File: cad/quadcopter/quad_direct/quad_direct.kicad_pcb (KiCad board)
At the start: 2 copper layers, 22.9 x 36.8 mm, 15 parts, among them SW1 SW_Push, SW2 SW_Push, U1 4pin_header, U2 8pin_header, U3 8pin_header, U4 3pin_header

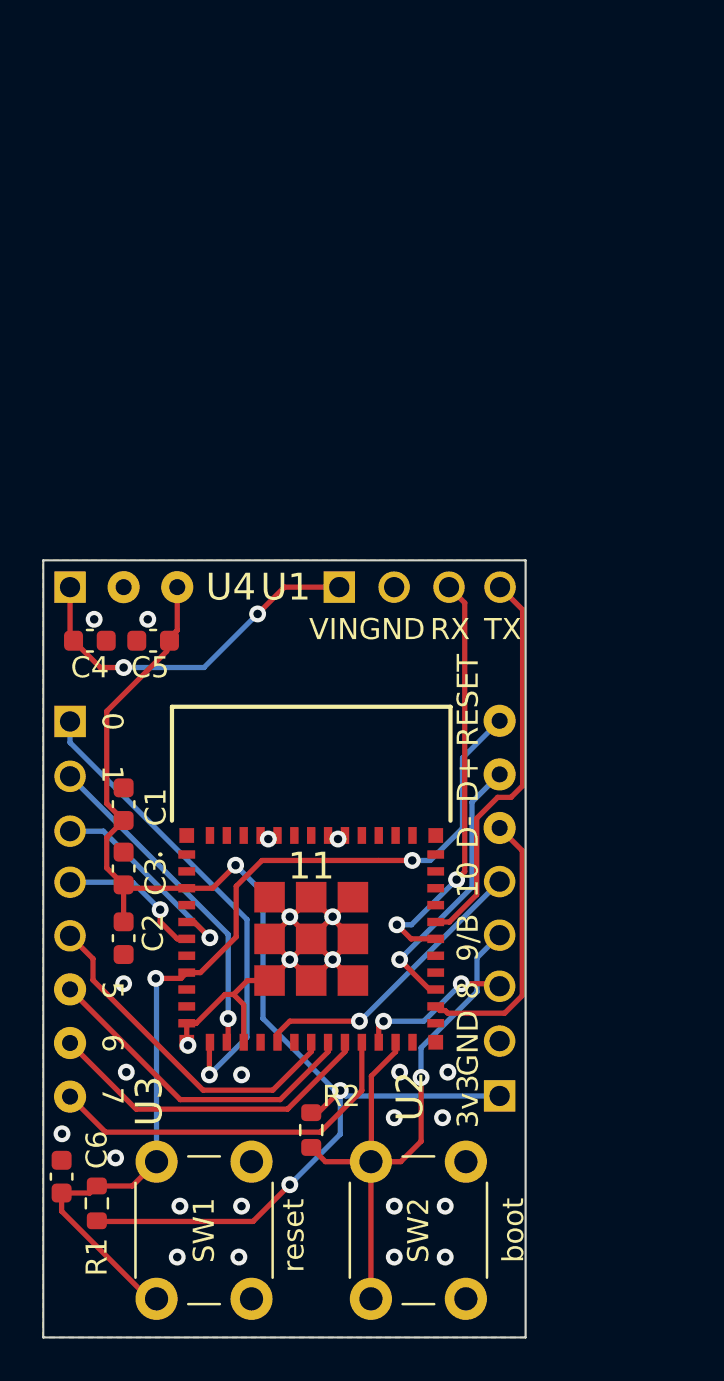
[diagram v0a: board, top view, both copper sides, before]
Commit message: Big progress saver
Signed-off-by: Andrew Wock <ajwock@gmail.com>
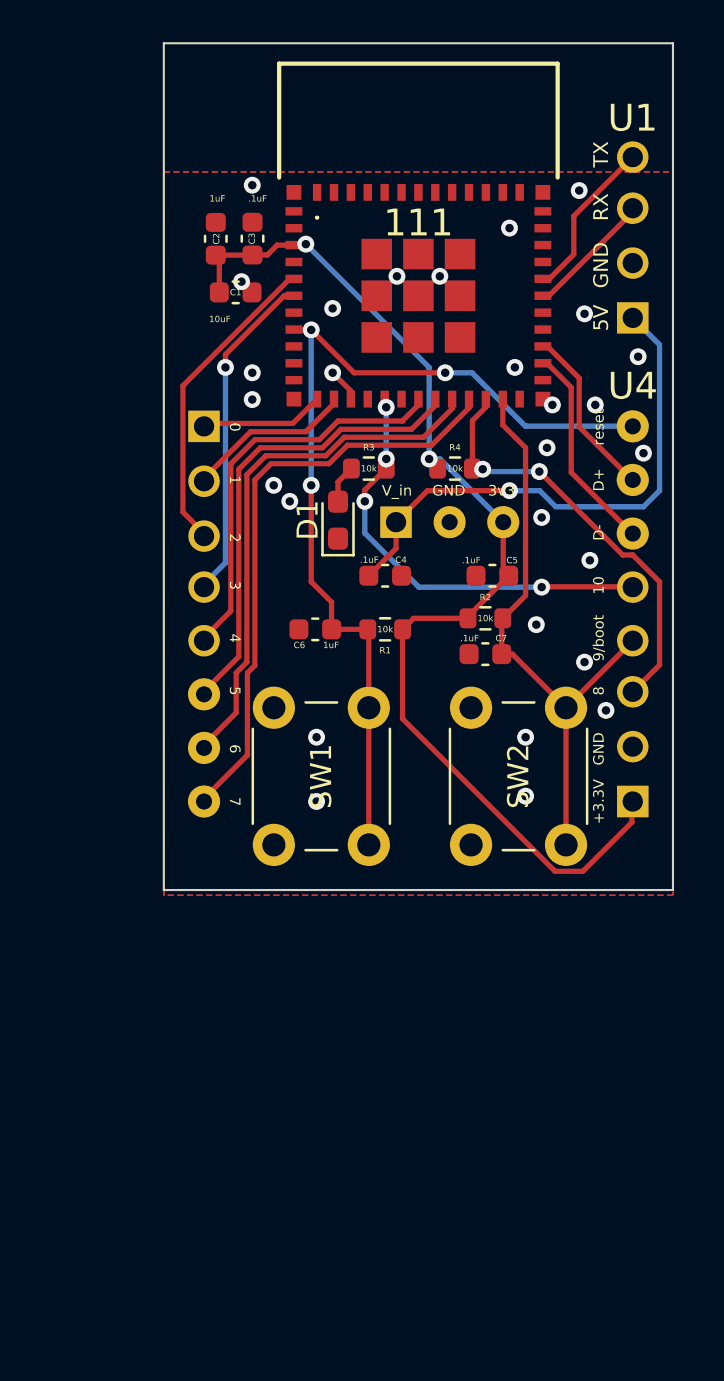
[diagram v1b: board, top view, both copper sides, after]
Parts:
- removed 11: ESP32-C3-MINI-1-H4X, Imported:ESP32C3MINI1H4X
- removed U3: 8pin_header, Imported:8-bb
- added 111: ESP32-C3-MINI-1-H4X, Imported:ESP32C3MINI1H4X, F.Cu at (165.1, 35.6)
- added C7: .1u, Capacitor_SMD:C_0603_1608Metric, F.Cu at (168.3, 55.2)
- added D1: LED, LED_SMD:LED_0603_1608Metric_Pad1.05x0.95mm_HandSolder, F.Cu at (161.3, 48.9)
- added R3: 10k, Resistor_SMD:R_0603_1608Metric, F.Cu at (162.8, 46.5)
- added R4: 10k, Resistor_SMD:R_0603_1608Metric, F.Cu at (166.8, 46.5)
- R1, R2: value R_US -> 10k
- U2: value 8pin_header -> esp32c3_boardout; footprint Imported:8-bb -> Imported:esp32c3_boardout
- moved C3 33.7 mm to (157.2, 35.6), turned to 90 degrees
- moved R1 30.4 mm to (163.5, 54.1), turned to 180 degrees
- moved C2 30.2 mm to (155.5, 35.6)
- moved SW1 29.8 mm to (162.8, 57.8), turned to -90 degrees
- moved SW2 29.5 mm to (172.1, 57.8), turned to -90 degrees
- moved C6 28.6 mm to (160.2, 54.1), turned to 180 degrees
- moved R2 25.6 mm to (168.3, 53.5), turned to 0 degrees
- moved C1 24.8 mm to (156.4, 38.1), turned to 0 degrees
- moved U2 20.9 mm to (152.4, 63.5), turned to 0 degrees
- moved U1 18.9 mm to (175.3, 39.3), turned to 90 degrees
- moved C5 16.4 mm to (168.6, 51.5)
- moved U4 15.8 mm to (164.0, 49.0)
- moved C4 14.3 mm to (163.5, 51.5)
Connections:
- U2 pad 1: +3V3 -> IO0
- U2 pad 2: GND -> IO1
- U2 pad 3: IO8 -> IO2
- U2 pad 4: IO9_BOOT -> IO3
- U2 pad 5: IO10 -> IO4
- U2 pad 6: IO18_USB_D- -> IO5
- U2 pad 7: IO19_USB_D+ -> IO6
- U2 pad 8: RESET -> IO7
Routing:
- net GND: track 30.7 -> 1.61 mm, vias 26 -> 28
- net IO0: track 22.5 -> 5.84 mm, vias 1 -> 0
- net UART_RX: track 20.2 -> 6.08 mm, vias 2 -> 0
- net IO8: track 7.38 -> 20.4 mm
- net UART_TX: track 18.8 -> 7.71 mm
- net IO7: track 17.6 -> 28.1 mm
- net IO6: track 15.9 -> 25.1 mm
- net IO3: track 6.98 -> 15.7 mm
- net +3V3: track 61.7 -> 53.1 mm, vias 3 -> 2
- net +5V: track 17.3 -> 25.5 mm, vias 2 -> 1
- net IO1: track 15.7 -> 7.84 mm, vias 1 -> 0
- net IO10: track 13.6 -> 20.5 mm, vias 1 -> 4
- net IO5: track 15.8 -> 22.1 mm
- net IO19_USB_D+: track 13.0 -> 8.19 mm, vias 1 -> 0
- net IO2: track 10.1 -> 14.8 mm, vias 1 -> 0
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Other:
- board size 22.9 x 36.8 mm -> 24.1 x 40.1 mm

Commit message: Makera setup
Signed-off-by: Andrew Wock <ajwock@gmail.com>
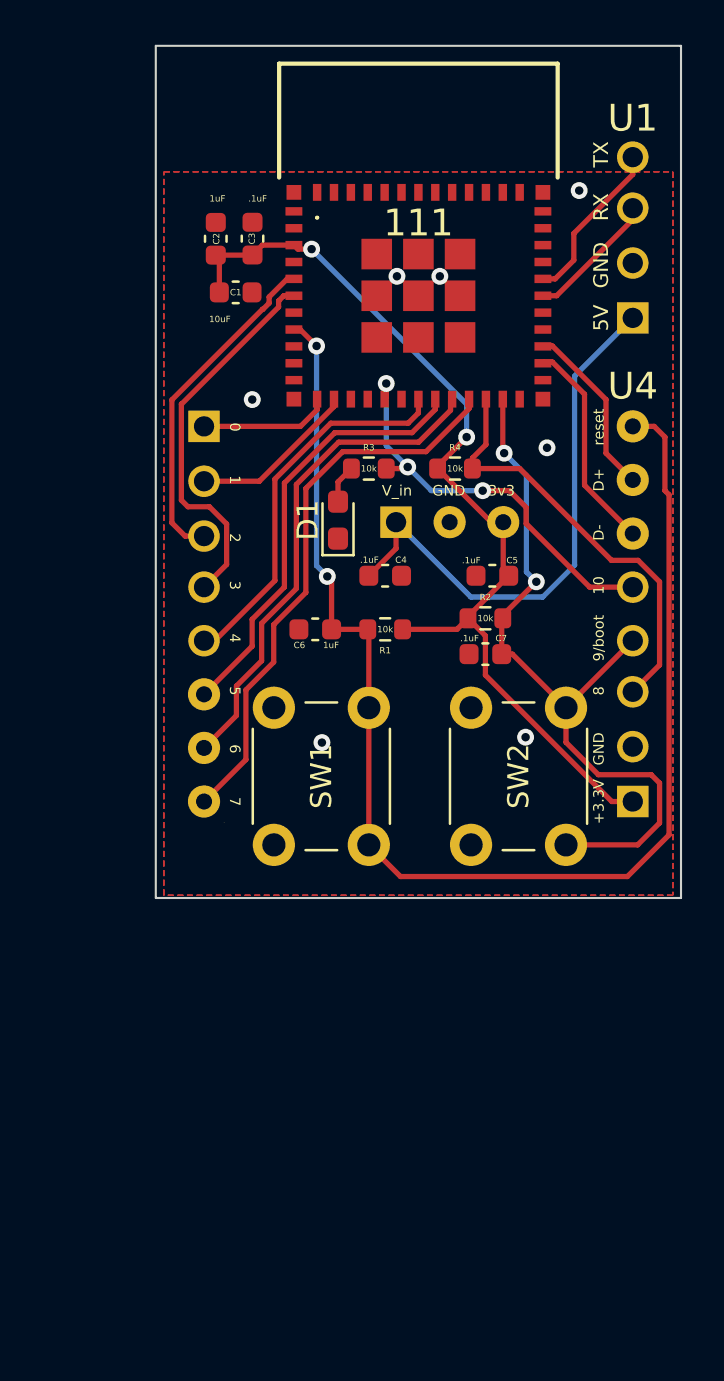
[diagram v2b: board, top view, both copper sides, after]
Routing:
- net RESET: track 44.5 -> 63.4 mm, vias 3 -> 2
- net IO9_BOOT: track 28.1 -> 35.6 mm, vias 0 -> 2
- net +3V3: track 53.1 -> 46.1 mm
- net IO3: track 15.7 -> 18.3 mm, vias 1 -> 0
- net GND: track 1.61 -> 0.00 mm, vias 28 -> 7
- net IO6: track 25.1 -> 23.6 mm
- net IO7: track 28.1 -> 26.6 mm
- net IO5: track 22.1 -> 20.7 mm
- net IO2: track 14.8 -> 15.9 mm
- net IO4: track 19.1 -> 18.1 mm
- net +5V: track 25.5 -> 26.5 mm, vias 1 -> 0
- net IO10: track 20.5 -> 19.7 mm, vias 4 -> 3
- net IO8: vias 2 -> 0
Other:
- board size 24.1 x 40.1 mm -> 24.9 x 40.4 mm
